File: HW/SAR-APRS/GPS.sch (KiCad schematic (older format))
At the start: 12 parts, among them J4 uFl, U10 NEO-M8, U11 EEPROM, U9 NEO_GPS_MODULE

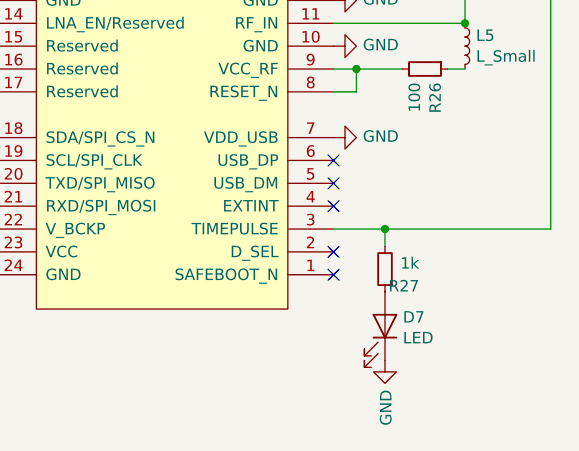
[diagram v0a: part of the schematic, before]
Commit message: schm and pcb update
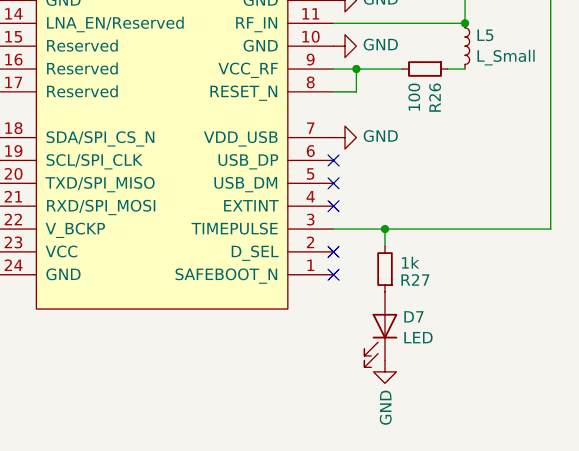
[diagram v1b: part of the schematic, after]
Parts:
- C23, C24, C25: footprint (none) -> Capacitors_SMD:C_0603
- L5: footprint (none) -> Inductors_SMD:L_0805
- R26, R27: footprint (none) -> Resistors_SMD:R_0603
- U9: footprint (none) -> Mlab_Pin_Headers:Straight_1x04
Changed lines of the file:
@@
 F 0 "U9" H 6025 3375 50  0000 C CNN
 F 1 "NEO_GPS_MODULE" H 6025 3284 50  0000 C CNN
-F 2 "" H 5525 3300 50  0001 C CNN
+F 2 "Mlab_Pin_Headers:Straight_1x04" H 5525 3300 50  0001 C CNN
 F 3 "" H 5525 3300 50  0001 C CNN
 	1    6025 3000
@@
 F 0 "C23" H 5342 2896 50  0000 L CNN
 F 1 "100nF" H 5342 2805 50  0000 L CNN
-F 2 "" H 5250 2850 50  0001 C CNN
+F 2 "Capacitors_SMD:C_0603" H 5250 2850 50  0001 C CNN
 F 3 "~" H 5250 2850 50  0001 C CNN
 	1    5250 2850
@@
 F 0 "R26" H 7909 4021 50  0000 L CNN
 F 1 "100" H 7909 3930 50  0000 L CNN
-F 2 "" H 7850 3975 50  0001 C CNN
+F 2 "Resistors_SMD:R_0603" H 7850 3975 50  0001 C CNN
 F 3 "~" H 7850 3975 50  0001 C CNN
 	1    7850 3975
@@
 F 0 "L5" H 8073 3921 50  0000 L CNN
 F 1 "L_Small" H 8073 3830 50  0000 L CNN
-F 2 "" H 8025 3875 50  0001 C CNN
+F 2 "Inductors_SMD:L_0805" H 8025 3875 50  0001 C CNN
 F 3 "~" H 8025 3875 50  0001 C CNN
 	1    8025 3875
@@
 F 0 "C25" H 5550 4950 50  0000 L CNN
 F 1 "100nF" H 5500 4875 50  0000 L CNN
-F 2 "" H 5425 4875 50  0001 C CNN
+F 2 "Capacitors_SMD:C_0603" H 5425 4875 50  0001 C CNN
 F 3 "~" H 5425 4875 50  0001 C CNN
 	1    5425 4875
@@
 F 0 "C24" H 3725 4075 50  0000 L CNN
 F 1 "100nF" H 3675 4000 50  0000 L CNN
-F 2 "" H 3600 4000 50  0001 C CNN
+F 2 "Capacitors_SMD:C_0603" H 3600 4000 50  0001 C CNN
 F 3 "~" H 3600 4000 50  0001 C CNN
 	1    3600 4000
@@
 AR Path="/5C995C89" Ref="R?"  Part="1"
 AR Path="/5C97B601/5C995C89" Ref="R27"  Part="1"
-F 0 "R27" H 7525 4925 50  0000 L CNN
+F 0 "R27" H 7475 4900 50  0000 L CNN
 F 1 "1k" H 7525 4825 50  0000 L CNN
-F 2 "" H 7675 4850 50  0001 C CNN
+F 2 "Resistors_SMD:R_0603" H 7675 4850 50  0001 C CNN
 F 3 "~" H 7675 4850 50  0001 C CNN
 	1    7675 4850

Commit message: PCB update
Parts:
- C23, C24, C25: footprint Capacitors_SMD:C_0603 -> Capacitors_SMD:C_0805
- C26: footprint (none) -> Capacitors_SMD:C_1210
- D7: footprint (none) -> LEDs:LED_0805
- R26, R27: footprint Resistors_SMD:R_0603 -> Resistors_SMD:R_0805
- U10: footprint (none) -> RF_GPS:ublox_NEO
- U11: footprint (none) -> IO:TSSOP-8_4.4x3mm_P0.65mm
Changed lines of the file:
@@
 F 0 "C23" H 5342 2896 50  0000 L CNN
 F 1 "100nF" H 5342 2805 50  0000 L CNN
-F 2 "Capacitors_SMD:C_0603" H 5250 2850 50  0001 C CNN
+F 2 "Capacitors_SMD:C_0805" H 5250 2850 50  0001 C CNN
 F 3 "~" H 5250 2850 50  0001 C CNN
 	1    5250 2850
@@
 F 0 "U10" H 6700 5190 50  0000 C CNN
 F 1 "NEO-M8" H 6700 5099 50  0000 C CNN
-F 2 "" H 6250 5375 50  0001 C CNN
+F 2 "RF_GPS:ublox_NEO" H 6250 5375 50  0001 C CNN
 F 3 "" H 6250 5375 50  0001 C CNN
 	1    6700 4275
@@
 F 0 "C26" H 5700 4900 50  0000 L CNN
 F 1 "10uF" H 5650 4800 50  0000 L CNN
-F 2 "" H 5600 4875 50  0001 C CNN
+F 2 "Capacitors_SMD:C_1210" H 5600 4875 50  0001 C CNN
 F 3 "~" H 5600 4875 50  0001 C CNN
 	1    5600 4875
@@
 F 0 "R26" H 7909 4021 50  0000 L CNN
 F 1 "100" H 7909 3930 50  0000 L CNN
-F 2 "Resistors_SMD:R_0603" H 7850 3975 50  0001 C CNN
+F 2 "Resistors_SMD:R_0805" H 7850 3975 50  0001 C CNN
 F 3 "~" H 7850 3975 50  0001 C CNN
 	1    7850 3975
@@
 F 0 "C25" H 5550 4950 50  0000 L CNN
 F 1 "100nF" H 5500 4875 50  0000 L CNN
-F 2 "Capacitors_SMD:C_0603" H 5425 4875 50  0001 C CNN
+F 2 "Capacitors_SMD:C_0805" H 5425 4875 50  0001 C CNN
 F 3 "~" H 5425 4875 50  0001 C CNN
 	1    5425 4875
@@
 F 0 "U11" H 3575 4975 60  0000 C CNN
 F 1 "EEPROM" H 4150 4950 60  0000 C CNN
-F 2 "" H 3825 4575 60  0001 C CNN
+F 2 "IO:TSSOP-8_4.4x3mm_P0.65mm" H 3825 4575 60  0001 C CNN
 F 3 "" H 3825 4575 60  0001 C CNN
 	1    3825 4575
@@
 F 0 "C24" H 3725 4075 50  0000 L CNN
 F 1 "100nF" H 3675 4000 50  0000 L CNN
-F 2 "Capacitors_SMD:C_0603" H 3600 4000 50  0001 C CNN
+F 2 "Capacitors_SMD:C_0805" H 3600 4000 50  0001 C CNN
 F 3 "~" H 3600 4000 50  0001 C CNN
 	1    3600 4000
@@
 F 0 "D7" V 7714 5178 50  0000 L CNN
 F 1 "LED" V 7623 5178 50  0000 L CNN
-F 2 "" H 7675 5100 50  0001 C CNN
+F 2 "LEDs:LED_0805" H 7675 5100 50  0001 C CNN
 F 3 "~" H 7675 5100 50  0001 C CNN
 	1    7675 5100
@@
 F 0 "R27" H 7475 4900 50  0000 L CNN
 F 1 "1k" H 7525 4825 50  0000 L CNN
-F 2 "Resistors_SMD:R_0603" H 7675 4850 50  0001 C CNN
+F 2 "Resistors_SMD:R_0805" H 7675 4850 50  0001 C CNN
 F 3 "~" H 7675 4850 50  0001 C CNN
 	1    7675 4850
